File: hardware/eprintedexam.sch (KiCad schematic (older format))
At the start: 60 parts, among them J1 Conn_01x04, J2 Conn_01x08, Q1 2N7002, Q10 2N7002, Q2 2N7002, Q3 2N7002, Q4 2N7002, Q5 2N7002, Q6 2N7002, Q7 2N7002, Q8 2N7002, Q9 2N7002, SW1 SW_Push, SW2 SW_Push, SW3 SW_Push, SW4 SW_Push, U1 AP1117-33, U2 ESP-12F

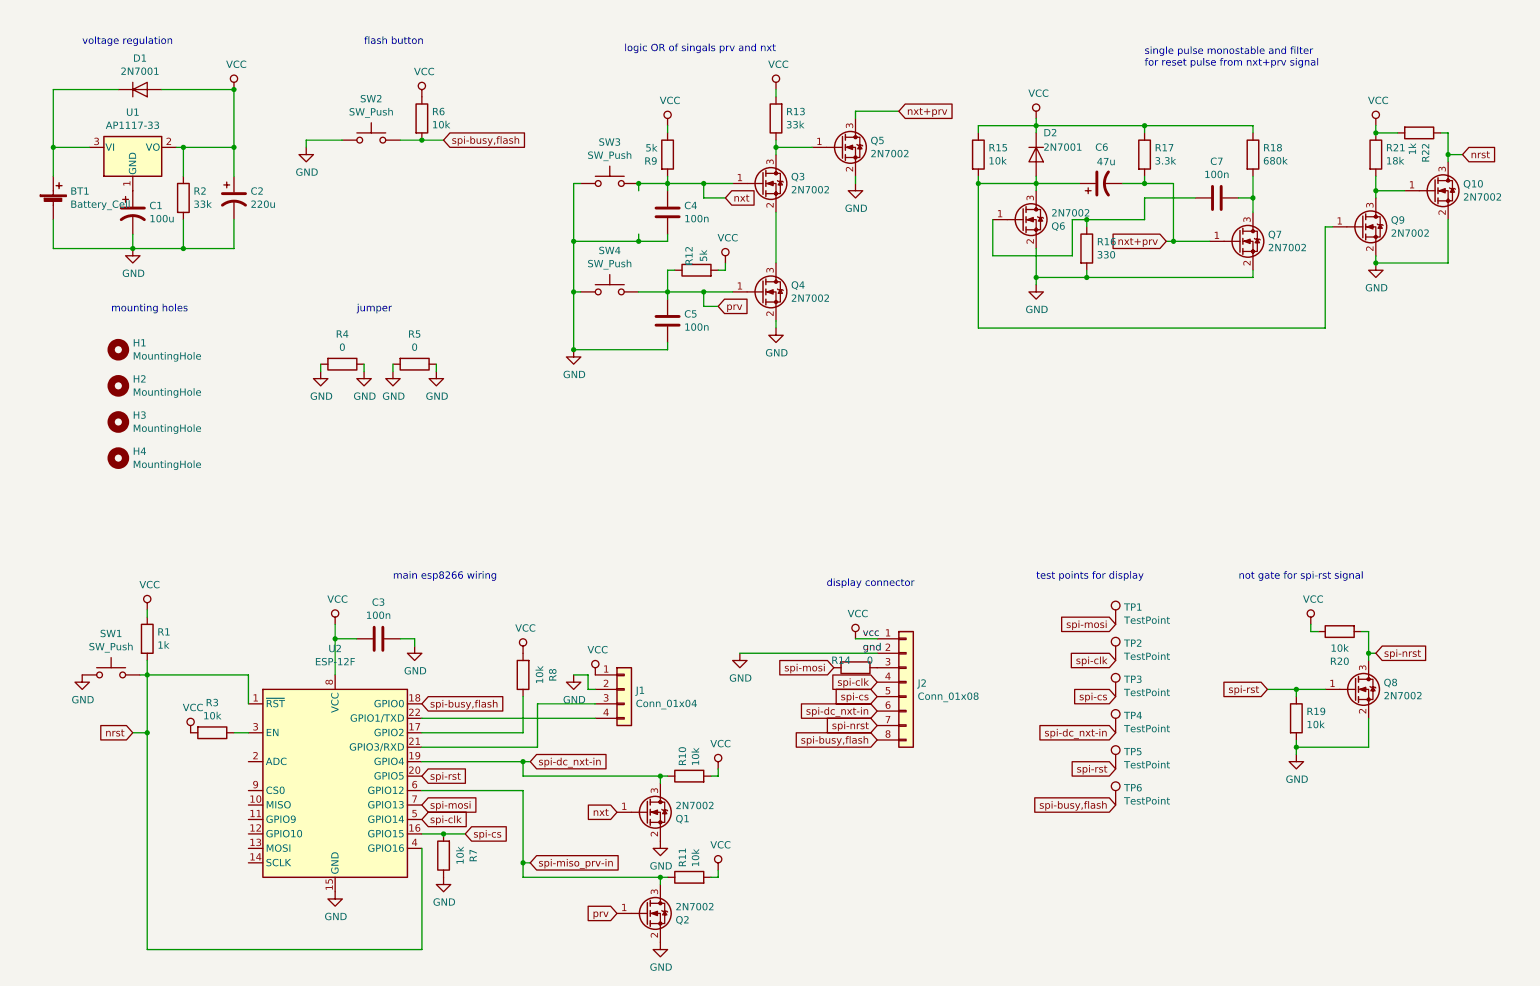
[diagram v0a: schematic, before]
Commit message: the hardware works
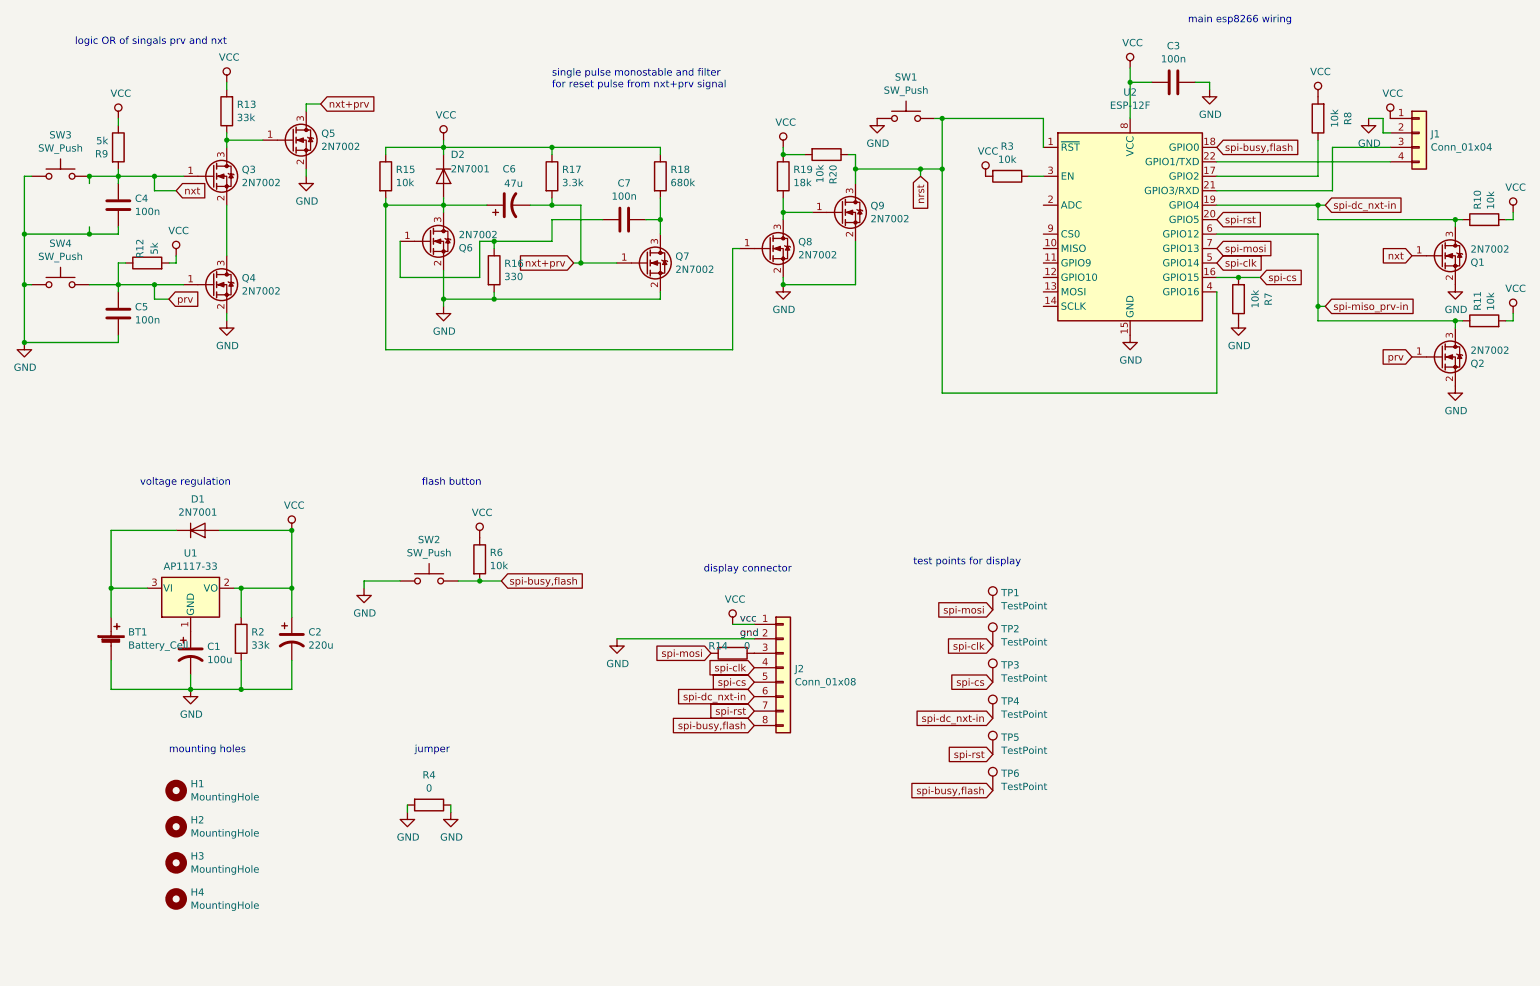
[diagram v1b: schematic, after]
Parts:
- removed Q8: 2N7002, Package_TO_SOT_SMD:SOT-23, symbol Transistor_FET:2N7002
- removed R1: 1k, Resistor_SMD:R_1206_3216Metric, symbol Device:R
- removed R19, R20: 10k, Resistor_SMD:R_1206_3216Metric, symbol Device:R
- removed R4: 0, Resistor_SMD:R_1206_3216Metric, symbol Device:R
- R20: renamed from R22; value 1k -> 10k
- renumbered Q9 to Q8, Q10 to Q9, R21 to R19, R5 to R4
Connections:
- net spi-nrst is gone; now on net spi-rst: J2.7 (Pin_7)
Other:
- note removed: "not gate for spi-rst signal"
- moved on the sheet: BT1, C1, C2, C3, C4, C5, C6, C7, D1, D2, H1, H2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
